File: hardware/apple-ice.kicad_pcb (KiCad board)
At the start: 2 copper layers, 100 x 77.7 mm, 77 parts, among them J1 TO_SP_DRIVE, J2 USB_B_Micro, J3 SPI_FLASH_PROG, P1 A2Bus-apple2, SW1 SW_Push, SW2 SW_Push, SW3 SW_Push, U1 SN74LVC8T245PW, U10 W25Q16JVSS, U2 SN74LVC8T245PW, U3 SN74LVC8T245PW, U4 SN74LVC8T245PW, U5 SN74LVC8T245PW, U6 ICE40HX1K-TQ144, U7 SN74LVC8T245PW, U8 MCP1703A-3302_SOT223, U9 MCP1703A-1202_SOT223, X1 ECS-2520MV-xxx-xx

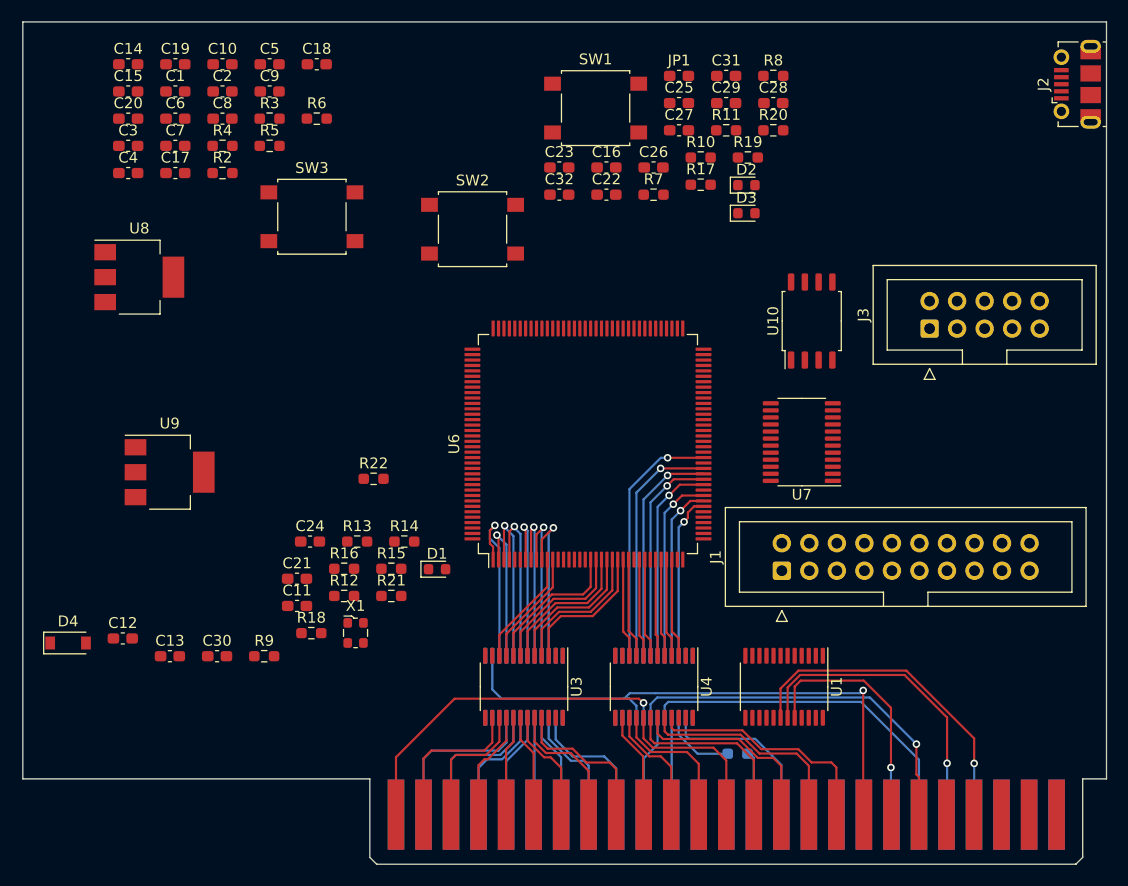
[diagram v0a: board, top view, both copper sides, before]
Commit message: Initial placement V2
Signed-off-by: Rangel Ivanov <rangelivanov88@gmail.com>
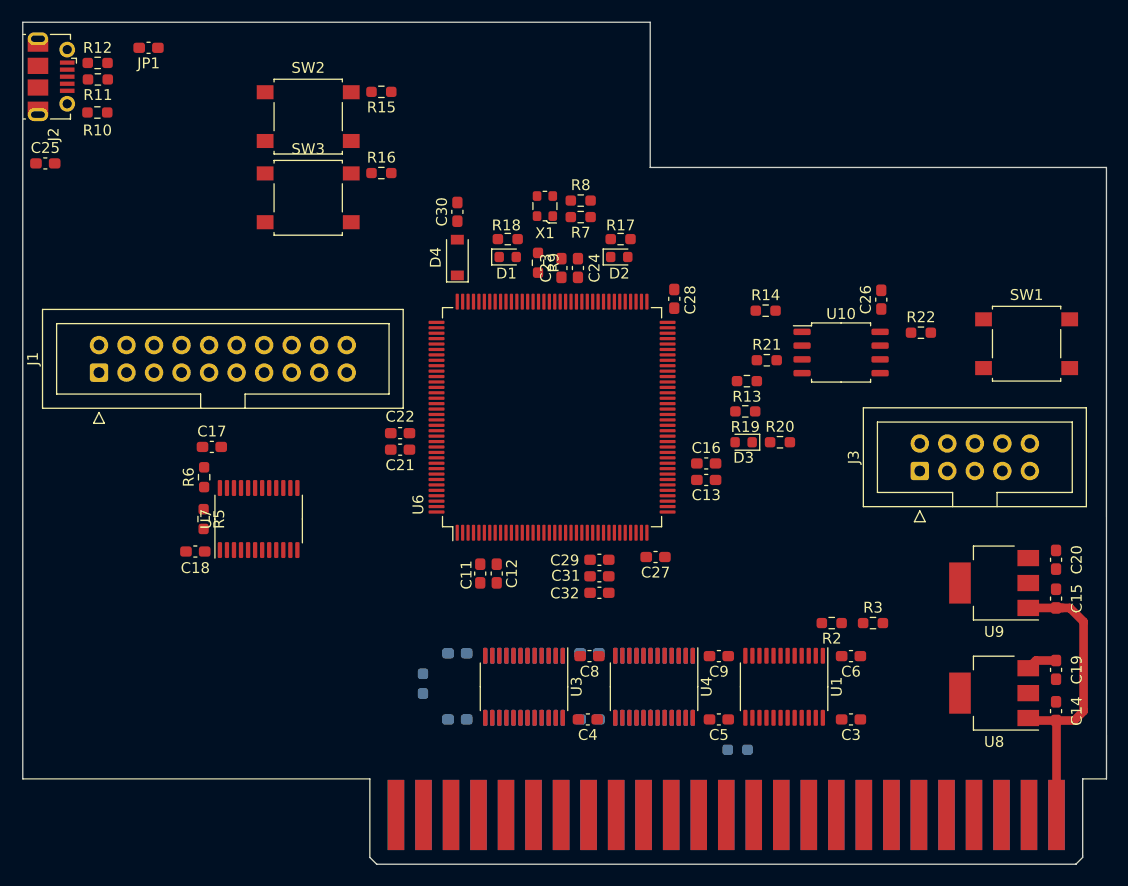
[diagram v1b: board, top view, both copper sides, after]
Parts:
- C1, C10, C2, C7, R4: moved to B.Cu
- moved C14 104.4 mm to (188.6, 95.2), turned to 90 degrees
- moved C19 98.6 mm to (188.6, 91.4), turned to 270 degrees
- moved C15 97.6 mm to (188.6, 84.9), turned to 90 degrees
- moved C20 94.8 mm to (188.6, 81.3), turned to 270 degrees
- moved J2 94.7 mm to (95.9, 36.7), turned to 270 degrees
- moved U8 87.7 mm to (182.9, 93.6), turned to 180 degrees
- moved C3 85.1 mm to (169.7, 96.0), turned to 180 degrees
- moved C6 79.7 mm to (169.7, 90.2), turned to 180 degrees
- moved U9 76.8 mm to (182.9, 83.4), turned to 180 degrees
- moved C5 73.3 mm to (157.5, 96.0), turned to 180 degrees
- moved R3 72.6 mm to (171.7, 87.1)
- moved R2 69.9 mm to (167.9, 87.1), turned to 180 degrees
- moved C2 67.1 mm to (145.5, 96.0)
- moved C9 66.6 mm to (157.5, 90.2), turned to 180 degrees
- moved C4 65.9 mm to (145.4, 96.0), turned to 180 degrees
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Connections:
- U6 pad 112: Net-(U6-Pad112) -> /PH0
- U6 pad 113: Net-(U6-Pad113) -> /PH1
- U6 pad 114: Net-(U6-Pad114) -> /PH2
- U6 pad 115: Net-(U6-Pad115) -> /PH3
- U6 pad 116: Net-(U6-Pad116) -> /~WREQ
- U6 pad 117: Net-(U6-Pad117) -> /SEL
- U6 pad 118: Net-(U6-Pad118) -> /~ENABLE
- U6 pad 119: Net-(U6-Pad119) -> /WRDATA
- U6 pad 120: Net-(U6-Pad120) -> /RDDATA_33
- U6 pad 121: Net-(U6-Pad121) -> /SENSE_33
- U6 pad 58: /PH0 -> Net-(U6-Pad58)
- U6 pad 60: /PH1 -> Net-(U6-Pad60)
- U6 pad 61: /PH2 -> Net-(U6-Pad61)
- U6 pad 62: /PH3 -> Net-(U6-Pad62)
- U6 pad 63: /~WREQ -> Net-(U6-Pad63)
- U6 pad 64: /SEL -> Net-(U6-Pad64)
- U6 pad 73: /~ENABLE -> Net-(U6-Pad73)
- U6 pad 74: /WRDATA -> Net-(U6-Pad74)
- U6 pad 75: /RDDATA_33 -> Net-(U6-Pad75)
- U6 pad 76: /SENSE_33 -> Net-(U6-Pad76)
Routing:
- net /RW: track 52.0 -> 0.00 mm, vias 1 -> 0
- net /~IOSTROBE: track 35.1 -> 0.66 mm, vias 1 -> 0
- net /~RES: track 32.0 -> 0.00 mm
- net /~IOSEL: track 31.9 -> 0.00 mm, vias 1 -> 0
- net Net-(P1-Pad29): track 30.9 -> 0.00 mm, vias 1 -> 0
- net +5V: track 0.00 -> 28.8 mm
- net Net-(P1-Pad30): track 28.6 -> 0.00 mm, vias 1 -> 0
- net /RW_33: track 23.4 -> 0.00 mm, vias 1 -> 0
- net Net-(P1-Pad32): track 22.9 -> 0.00 mm, vias 1 -> 0
- net /~IOSEL_33: track 22.2 -> 0.00 mm, vias 1 -> 0
- net /A15: track 22.0 -> 0.00 mm
- net /~IOSTROBE_33: track 20.9 -> 0.00 mm, vias 1 -> 0
- net /A14: track 20.4 -> 0.00 mm
- net /~DEVSEL_33: track 19.9 -> 0.00 mm, vias 1 -> 0
- net /~RES_33: track 18.8 -> 0.00 mm, vias 1 -> 0
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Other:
- outline, holes or cut-outs redrawn
